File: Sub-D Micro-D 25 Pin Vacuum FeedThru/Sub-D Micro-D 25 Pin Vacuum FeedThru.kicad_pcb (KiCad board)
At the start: 2 copper layers, 53 x 53 mm, 6 parts, among them J1 DB25_Male, J2 DB25_Male, J3 DB25_Male, J4 DB25_Male, J5 DB25_Male, J6 DB25_Male

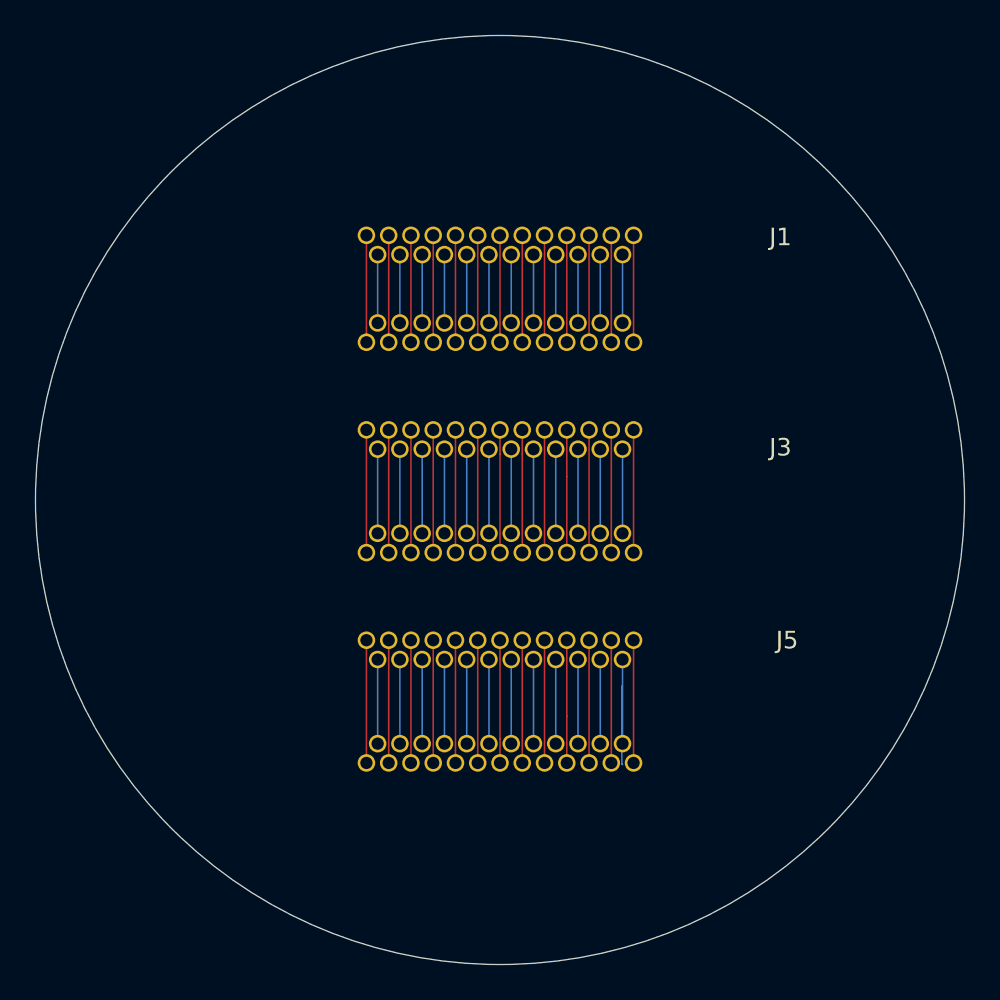
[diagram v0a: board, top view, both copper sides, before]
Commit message: Update Gerber
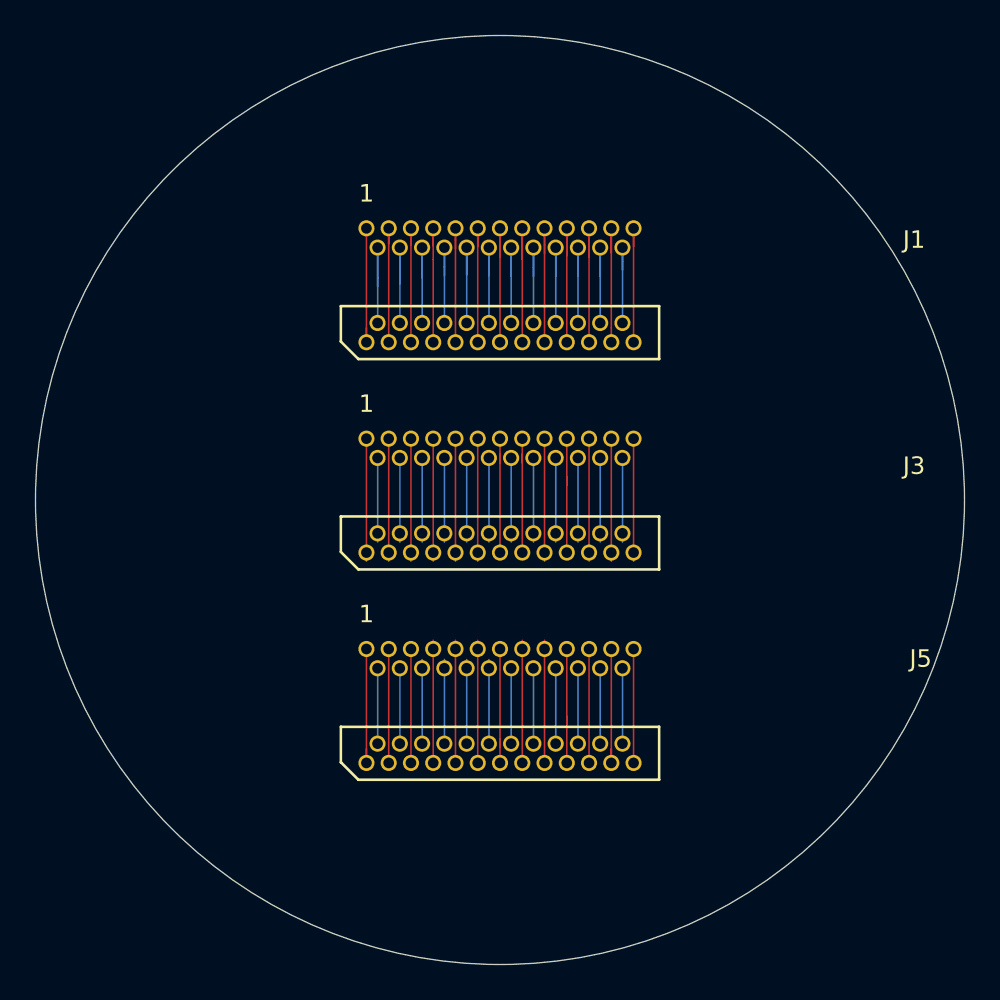
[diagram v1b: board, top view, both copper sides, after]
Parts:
- J1, J2, J3, J4, J5, J6: footprint Connector:MicroD_25Pin_NorComp -> Connector:Norcomp-380-025-113L001-microd_Updated
- moved J3 7.69 mm to (0.00, -2.95)
- moved J5 7.69 mm to (0.00, 9.05)
- moved J2 7.64 mm to (0.00, -9.55)
- moved J4 7.64 mm to (0.00, 2.45)
- moved J6 7.64 mm to (0.00, 14.4)
- moved J1 7.62 mm to (0.00, -14.9)
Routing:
- net Net-(J5-Pad25): track 9.31 -> 4.80 mm
- net Net-(J1-Pad14): track 3.90 -> 6.11 mm
- net Net-(J1-Pad15): track 3.90 -> 5.95 mm
- net Net-(J1-Pad8): track 6.10 -> 7.87 mm
- net Net-(J1-Pad16): track 3.90 -> 5.62 mm
- net Net-(J1-Pad22): track 3.90 -> 5.57 mm
- net Net-(J1-Pad20): track 3.90 -> 5.56 mm
- net Net-(J1-Pad24): track 3.90 -> 5.55 mm
- net Net-(J1-Pad21): track 3.90 -> 5.55 mm
- net Net-(J1-Pad7): track 6.10 -> 7.74 mm
- net Net-(J1-Pad23): track 3.90 -> 5.53 mm
- net Net-(J1-Pad11): track 6.10 -> 7.73 mm
- net Net-(J1-Pad19): track 3.90 -> 5.50 mm
- net Net-(J1-Pad17): track 3.90 -> 5.50 mm
- net Net-(J1-Pad18): track 3.90 -> 5.46 mm
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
